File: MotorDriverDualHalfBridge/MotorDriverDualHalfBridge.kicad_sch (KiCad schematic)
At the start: 41 parts, among them J1 Battery Terminal +, J2 Battery Terminal -, J3 Motor Battery Connection, J4 Motor Load Connection, J5 Conn_01x02_Male, J6 Conn_01x02_Male, K1 G8PM, Q1 IAUA250N04S6N005, Q2 IAUA250N04S6N005, Q3 Q_NMOS_DGS, U1 2ED21824S06J, U2 TLI4871

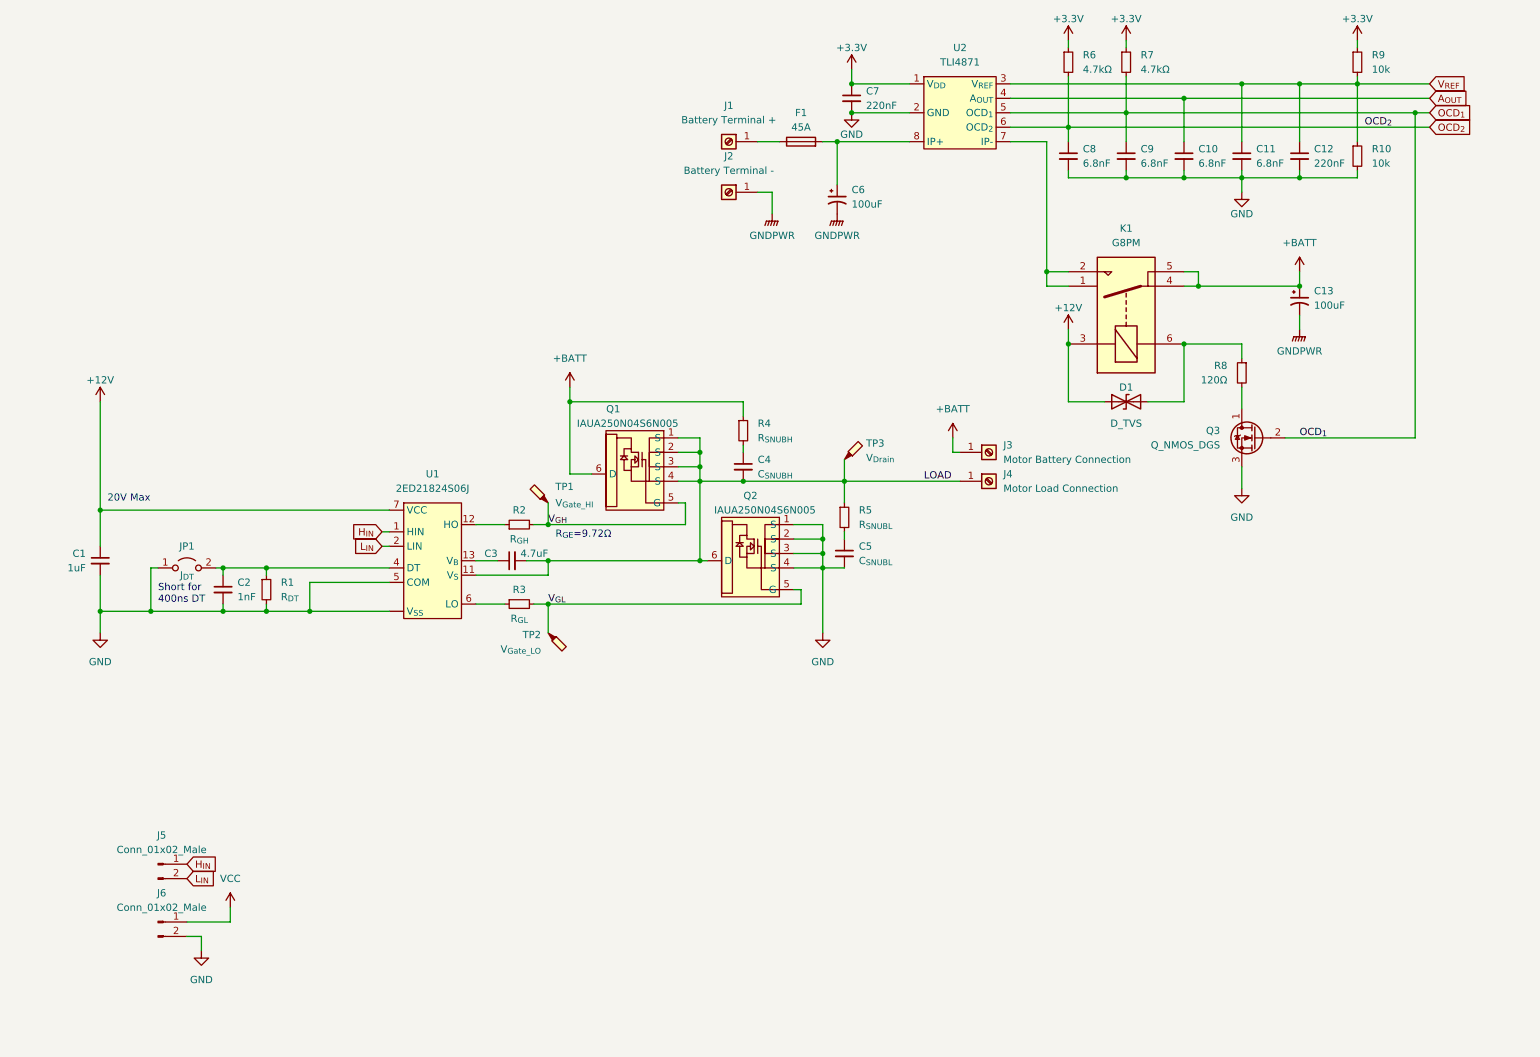
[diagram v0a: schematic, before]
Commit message: PCB V0.1
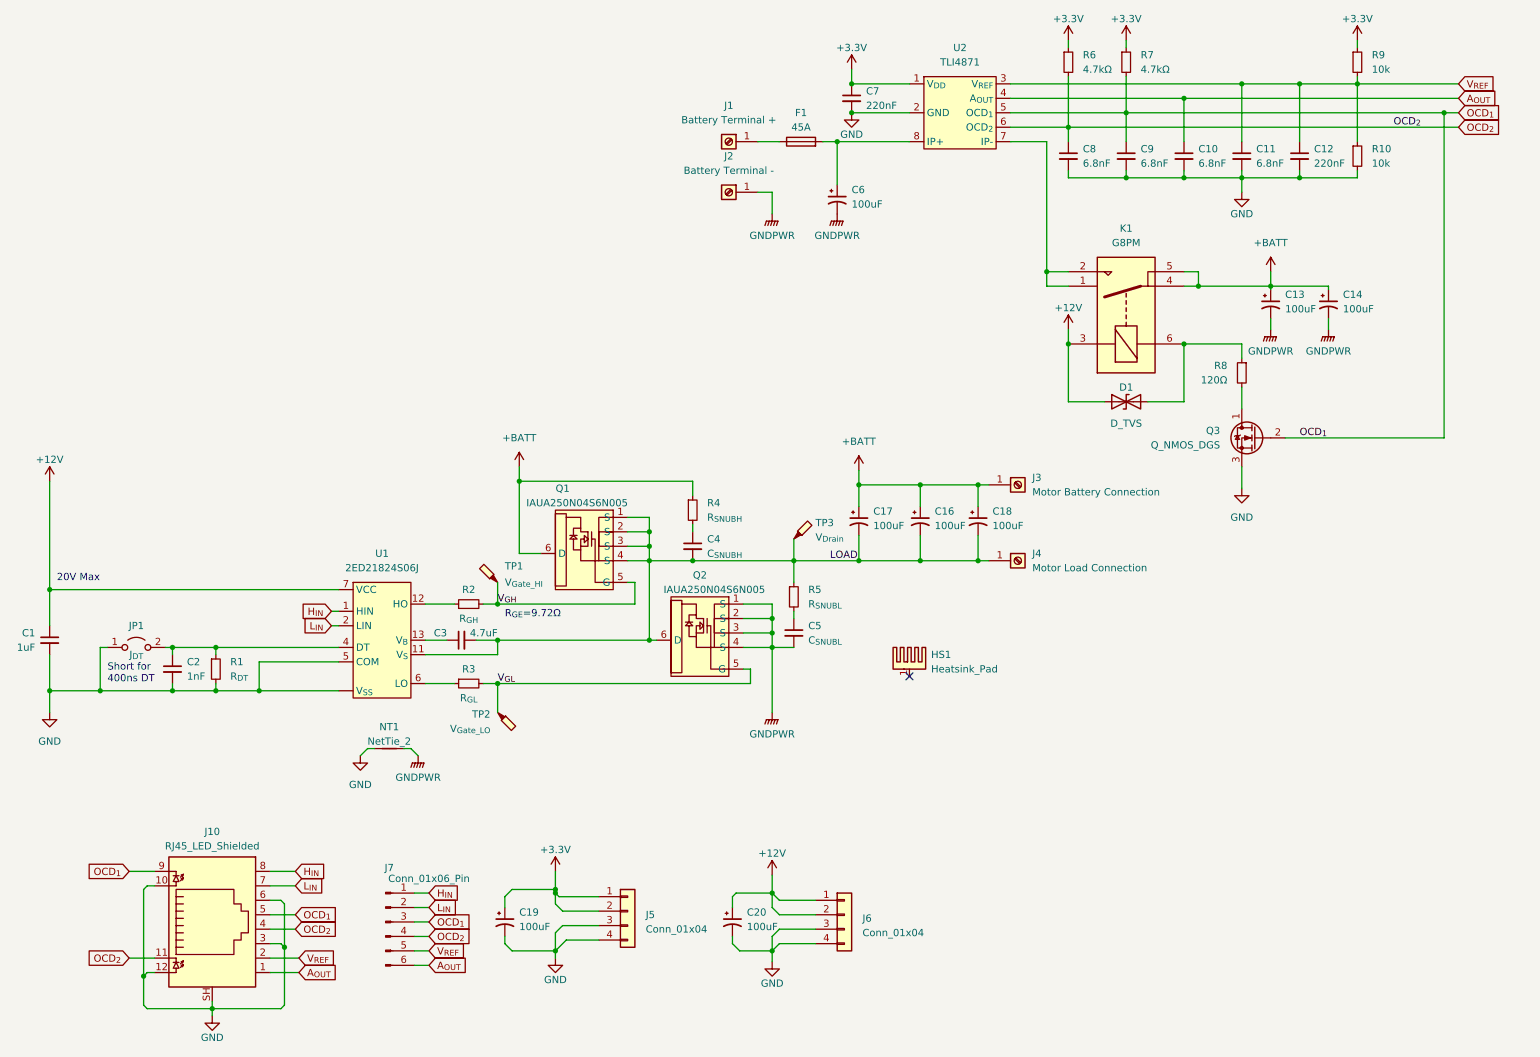
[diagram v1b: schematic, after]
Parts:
- removed J5, J6: Conn_01x02_Male, Connector_PinHeader_1.27mm:PinHeader_1x02_P1.27mm_Vertical, symbol Connector:Conn_01x02_Male
- added C14: 100uF, Capacitor_SMD:CP_Elec_10x14.3, symbol Device:C_Polarized_Small_US
- added C16, C17, C18, C19, C20: 100uF, Capacitor_SMD:CP_Elec_6.3x5.4_Nichicon, symbol Device:C_Polarized_Small_US
- added HS1: Heatsink_Pad, Library:HSB25-282810, symbol Mechanical:Heatsink_Pad
- added J10: RJ45_LED_Shielded, Connector_RJ:RJ45_Amphenol_RJHSE538X, symbol Connector:RJ45_LED_Shielded
- added J5, J6: Conn_01x04, Connector_JST:JST_EH_B4B-EH-A_1x04_P2.50mm_Vertical, symbol Connector_Generic:Conn_01x04
- added J7: Conn_01x06_Pin, Connector_PinHeader_1.27mm:PinHeader_1x06_P1.27mm_Vertical, symbol Connector:Conn_01x06_Pin
- added NT1: NetTie_2, NetTie:NetTie-2_SMD_Pad2.0mm, symbol Device:NetTie_2
- C13, C6: footprint Capacitor_SMD:CP_Elec_5x4.4 -> Capacitor_SMD:CP_Elec_10x14.3
- F1: footprint Fuse:Fuseholder_Clip-5x20mm_Bel_FC-203-22_Lateral_P17.80x5.00mm_D1.17mm_Horizontal -> Fuse:Fuseholder_Blade_Mini_Keystone_3568
- Q1, Q2: footprint IFX-PG-HSOF-5-1-V:IFX-PG-HSOF-5-1-V -> Library:IAUA250N04S6N005AUMA1
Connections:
- net +12V: now also C20.1, J6.1 (Pin_1), J6.2 (Pin_2)
- net +3.3V: now also C19.1, J5.1 (Pin_1), J5.2 (Pin_2)
- net +BATT: now also C14.1, C16.1, C17.1, C18.1
- net A_{OUT}: now also J10.1, J7.6 (Pin_6)
- net GND: now also C19.2, C20.2, J10.10, J10.12, J10.3, J10.6, J10.SH, J5.3 (Pin_3), J5.4 (Pin_4), J6.3 (Pin_3), J6.4 (Pin_4), NT1.1; no longer C5.2, Q2.1 (S), Q2.2 (S), Q2.3 (S), Q2.4 (S)
- net GNDPWR: now also C5.2, Q2.1 (S), Q2.2 (S), Q2.3 (S), Q2.4 (S), C14.2, NT1.2
- net H_{IN}: now also J10.8, J7.1 (Pin_1)
- net LOAD: now also C16.2, C17.2, C18.2
- net L_{IN}: now also J10.7, J7.2 (Pin_2)
- net OCD_{1}: now also J10.5, J10.9, J7.3 (Pin_3)
- net OCD_{2}: now also J10.11, J10.4, J7.4 (Pin_4)
- net V_{REF}: now also J10.2, J7.5 (Pin_5)
- no-connect marks 0 -> 1
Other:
- moved on the sheet: C1, C13, C2, C3, C4, C5, J3, J4, JP1, Q1, Q2, R1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

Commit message: Updated Schematic
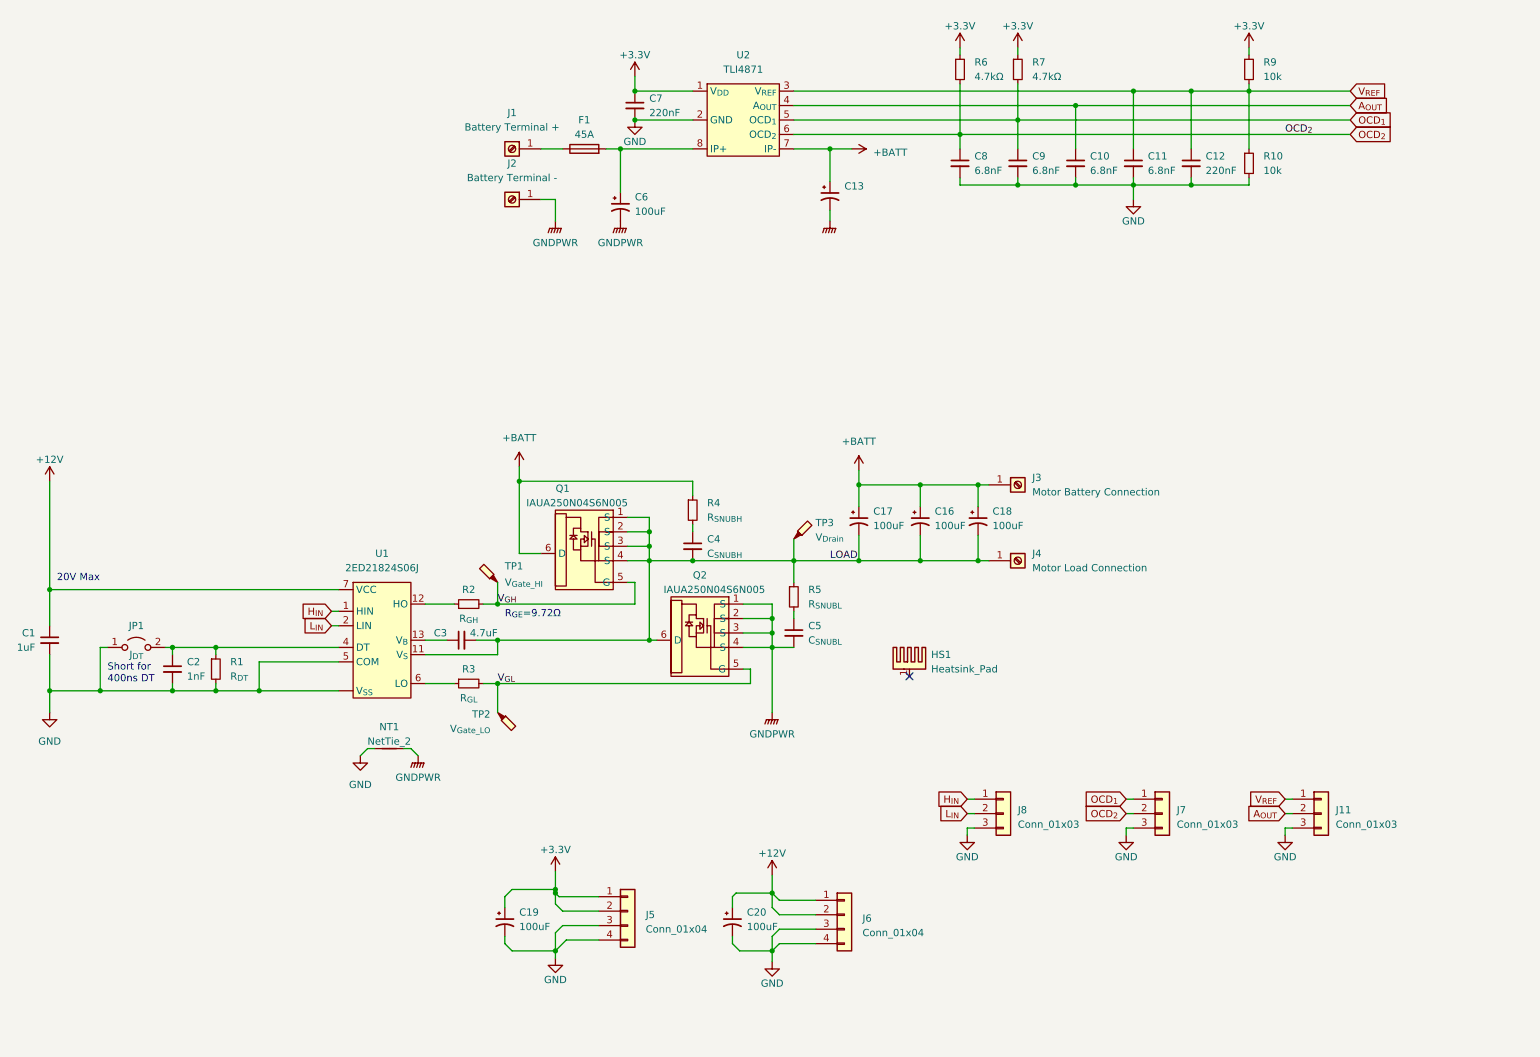
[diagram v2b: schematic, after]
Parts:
- removed C14: 100uF, Capacitor_SMD:CP_Elec_10x14.3, symbol Device:C_Polarized_Small_US
- removed D1: D_TVS, Diode_SMD:D_SMF, symbol Device:D_TVS
- removed J10: RJ45_LED_Shielded, Connector_RJ:RJ45_Amphenol_RJHSE538X, symbol Connector:RJ45_LED_Shielded
- removed J7: Conn_01x06_Pin, Connector_PinHeader_1.27mm:PinHeader_1x06_P1.27mm_Vertical, symbol Connector:Conn_01x06_Pin
- removed K1: G8PM, Library:G8PM1AW7RDC12, symbol MyLibrary:G8PM
- removed Q3: Q_NMOS_DGS, Package_TO_SOT_THT:TO-220F-3_Vertical, symbol Device:Q_NMOS_DGS
- removed R8: 120Ω, Resistor_SMD:R_0603_1608Metric_Pad0.98x0.95mm_HandSolder, symbol Device:R_Small
- added J11, J7, J8: Conn_01x03, Library:MOLEX_2078430003_L1NK_250_3-PIN, symbol Connector_Generic:Conn_01x03
- J5, J6: footprint Connector_JST:JST_EH_B4B-EH-A_1x04_P2.50mm_Vertical -> Library:MOLEX_2078430004_L1NK_250_4-PIN
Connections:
- net +BATT: now also U2.7 (IP-)
- net A_{OUT}: now also J11.2 (Pin_2)
- net GND: now also J11.3 (Pin_3), J7.3 (Pin_3), J8.3 (Pin_3)
- net H_{IN}: now also J8.1 (Pin_1)
- net L_{IN}: now also J8.2 (Pin_2)
- net OCD_{1}: now also J7.1 (Pin_1)
- net OCD_{2}: now also J7.2 (Pin_2)
- net V_{REF}: now also J11.1 (Pin_1)
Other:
- moved on the sheet: C10, C11, C12, C13, C6, C7, C8, C9, F1, J1, J2, R10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
